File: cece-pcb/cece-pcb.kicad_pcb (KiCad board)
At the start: 2 copper layers, 64 x 90 mm, 52 parts, among them J1 SERIAL, J2 HTU21D, J3 Li-Ion Battery, J4 VAC, K1 SANYOU_SRD_Form_C, Q1 Q_NPN, Q2 Q_NPN, SW1 RES, U1 ESP-12F, U2 MCP73811T-420I-OT, U3 TLV75533PDBV

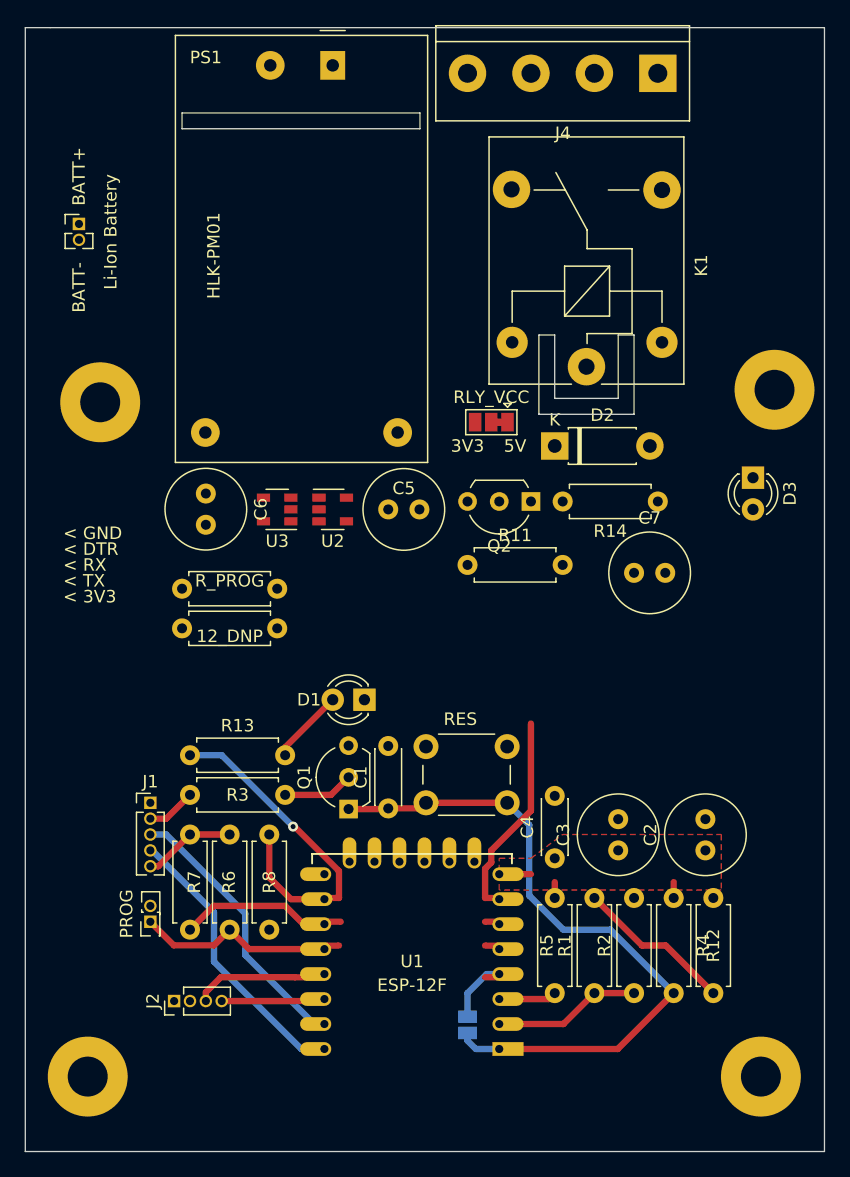
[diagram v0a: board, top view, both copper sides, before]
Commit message: Finish first board revision
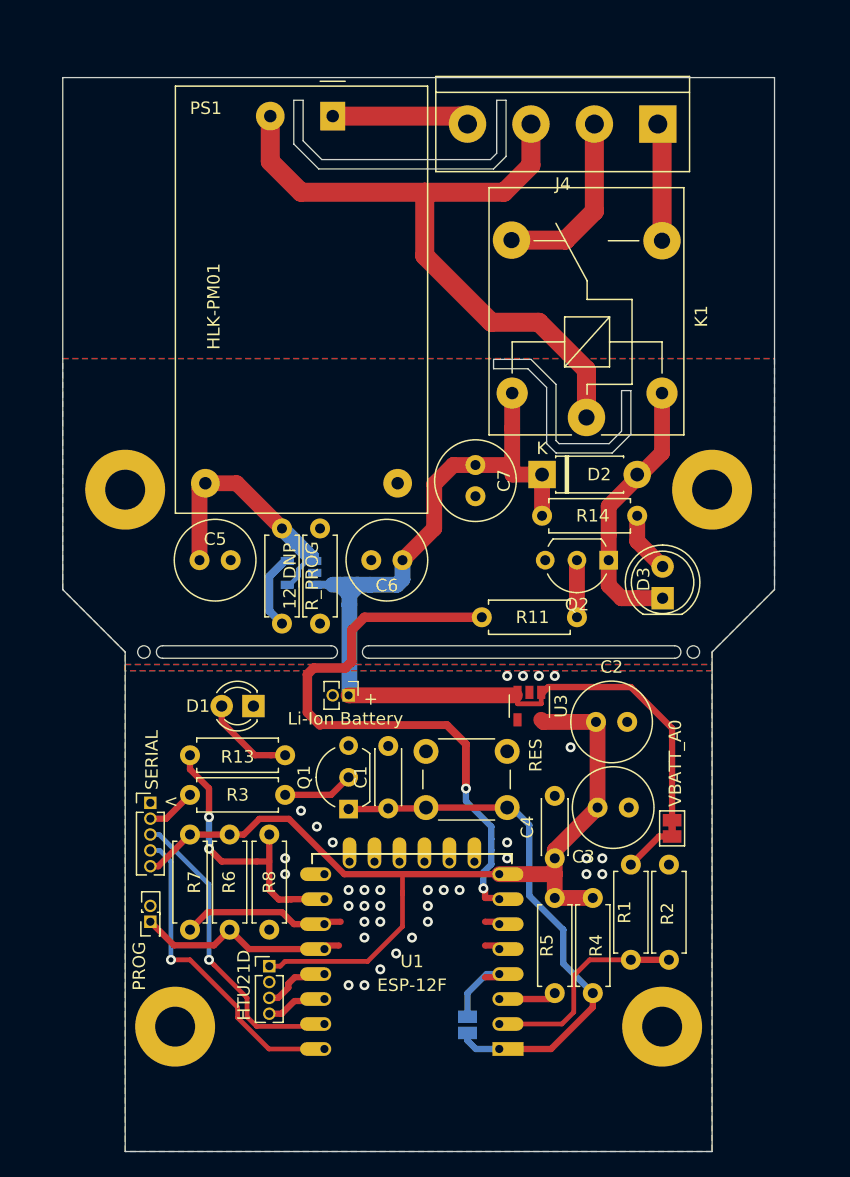
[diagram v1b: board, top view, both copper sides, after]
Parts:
- removed JP12: RLY_VCC, Jumper:SolderJumper-3_P1.3mm_Bridged12_Pad1.0x1.5mm
- removed R12: 100k, Resistor_THT:R_Axial_DIN0207_L6.3mm_D2.5mm_P7.62mm_Horizontal
- added JP2: VBATT_A0, Jumper:SolderJumper-2_P1.3mm_Bridged_Pad1.0x1.5mm, F.Cu at (161.8, 94.1)
- D3: footprint LED_THT:LED_D3.0mm -> LED_THT:LED_D5.0mm
- U2: moved to B.Cu
- moved J3 43.5 mm to (135.9, 83.5), turned to 270 degrees
- moved U3 25.6 mm to (150.4, 84.3), turned to 270 degrees
- moved C6 16.6 mm to (140.2, 72.6), turned to 180 degrees
- moved C5 15.6 mm to (124.0, 72.6)
- moved C7 15.4 mm to (146.1, 65.0), turned to 270 degrees
- moved C2 13.5 mm to (155.7, 85.6), turned to 0 degrees
- moved D3 12.1 mm to (161.0, 75.7), turned to 90 degrees
- moved R10 11.4 mm to (133.6, 77.7), turned to 90 degrees
- moved R11 9.71 mm to (154.2, 77.2), turned to 180 degrees
- moved H3 9.43 mm to (165.0, 67.0)
- moved D1 8.90 mm to (128.3, 84.3)
- moved H4 8.86 mm to (161.0, 110.0)
- moved J2 8.12 mm to (129.5, 105.2), turned to 0 degrees
- moved H2 8.06 mm to (122.0, 110.0)
- moved R9 8.01 mm to (130.6, 70.1), turned to 270 degrees
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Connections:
- C7 pad 1: Net-(C7-Pad1) -> +BATT
- D2 pad 1: Net-(C7-Pad1) -> +BATT
- J4 pad 1: /NC -> /NO
- J4 pad 2: /NO -> /NC
- K1 pad 5: Net-(C7-Pad1) -> +BATT
- NT1 pad 1: (no net) -> /ESP-12_common/D0
- NT2 pad 1: (no net) -> /ESP-12_common/D5|SCK
- NT3 pad 1: (no net) -> /ESP-12_common/D6|MISO
- NT8 pad 2: (no net) -> /ESP-12_common/D3
- NT9 pad 2: (no net) -> /ESP-12_common/D4
- R14 pad 2: Net-(C7-Pad1) -> +BATT
- U1 pad 17: (no net) -> Net-(U1-Pad17)
- U1 pad 18: (no net) -> Net-(U1-Pad18)
- U1 pad 19: (no net) -> Net-(U1-Pad19)
- U1 pad 20: (no net) -> Net-(U1-Pad20)
- U1 pad 21: (no net) -> Net-(U1-Pad21)
- U1 pad 22: (no net) -> Net-(U1-Pad22)
- U3 pad 4: (no net) -> Net-(U3-Pad4)
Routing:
- net +BATT: track 0.00 -> 82.4 mm
- net +3V3: track 12.5 -> 75.2 mm
- net /C: track 0.00 -> 55.4 mm
- net /RLY: track 15.5 -> 47.6 mm, vias 0 -> 2
- net Net-(D2-Pad2): track 0.00 -> 21.9 mm
- net +5V: track 0.00 -> 20.9 mm
- net /NC: track 0.00 -> 14.6 mm
- net /LN: track 0.00 -> 11.1 mm
- net /ESP-12_common/RST: track 55.1 -> 44.4 mm
- net /NO: track 0.00 -> 9.48 mm
- net /ESP-12_common/A0: track 12.7 -> 4.24 mm
- net Net-(R10-Pad1): track 0.00 -> 6.15 mm
- net /ESP-12_common/D8: track 18.0 -> 12.4 mm, vias 1 -> 2
- net /ESP-12_common/ADC: track 11.8 -> 17.4 mm
- net /HTU_SDA: track 8.32 -> 2.91 mm
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- added copper zone on B.Cu, net GND
- added copper zone on F.Cu, net GND
- removed copper zone on F.Cu, net +3V3
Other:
- board size 64 x 90 mm -> 57 x 86 mm
- board text added: "+"
- board text added: "<"
- board text removed: "3V3"
- board text removed: "5V"
- board text removed: "< 3V3"
- board text removed: "< DTR"
- board text removed: "< GND"
- board text removed: "< RX"
- board text removed: "< TX"
- board text removed: "BATT+"
- board text removed: "BATT-"
